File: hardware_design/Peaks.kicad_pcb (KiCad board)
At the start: 2 copper layers, 86.4 x 69.8 mm, 54 parts, among them J3 Eurorack Power, J8 Conn_01x07, Q1 2N3904, Q2 2N3904, U1 TL074, U2 Bluepill, U3 78l05

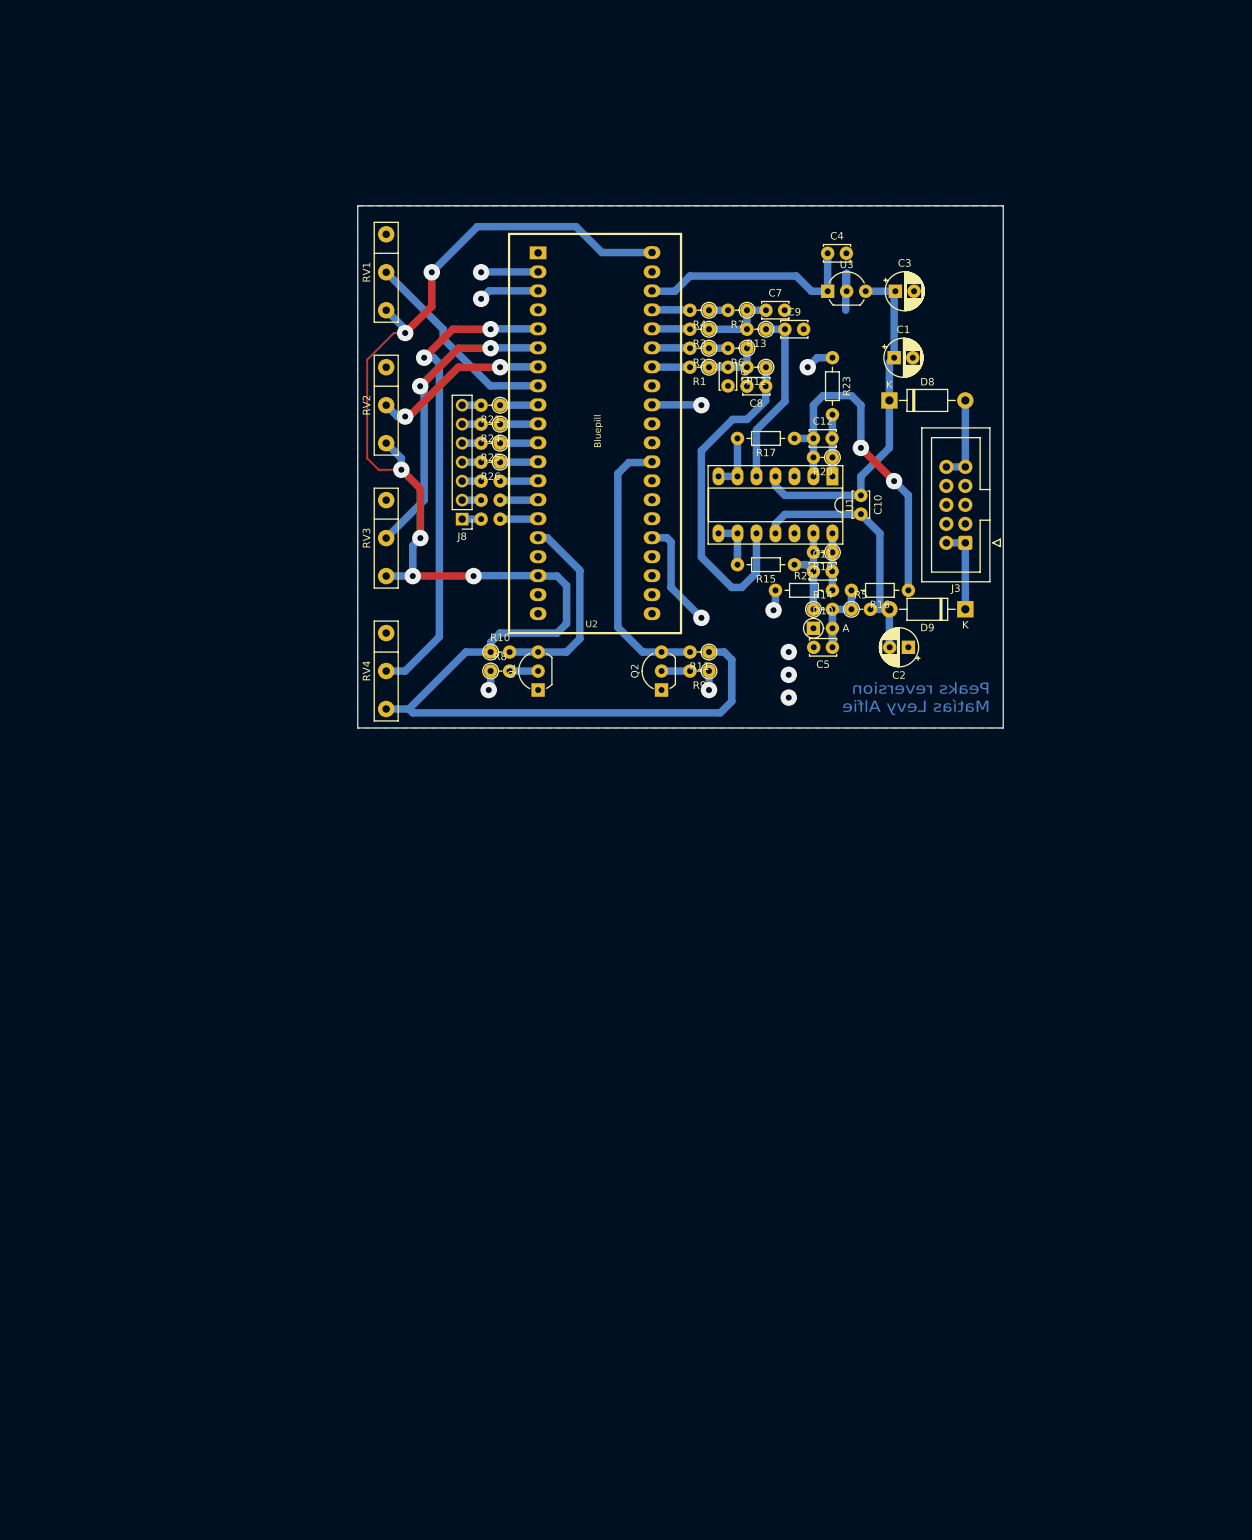
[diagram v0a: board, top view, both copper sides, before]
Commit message: update my KOSMO adaption
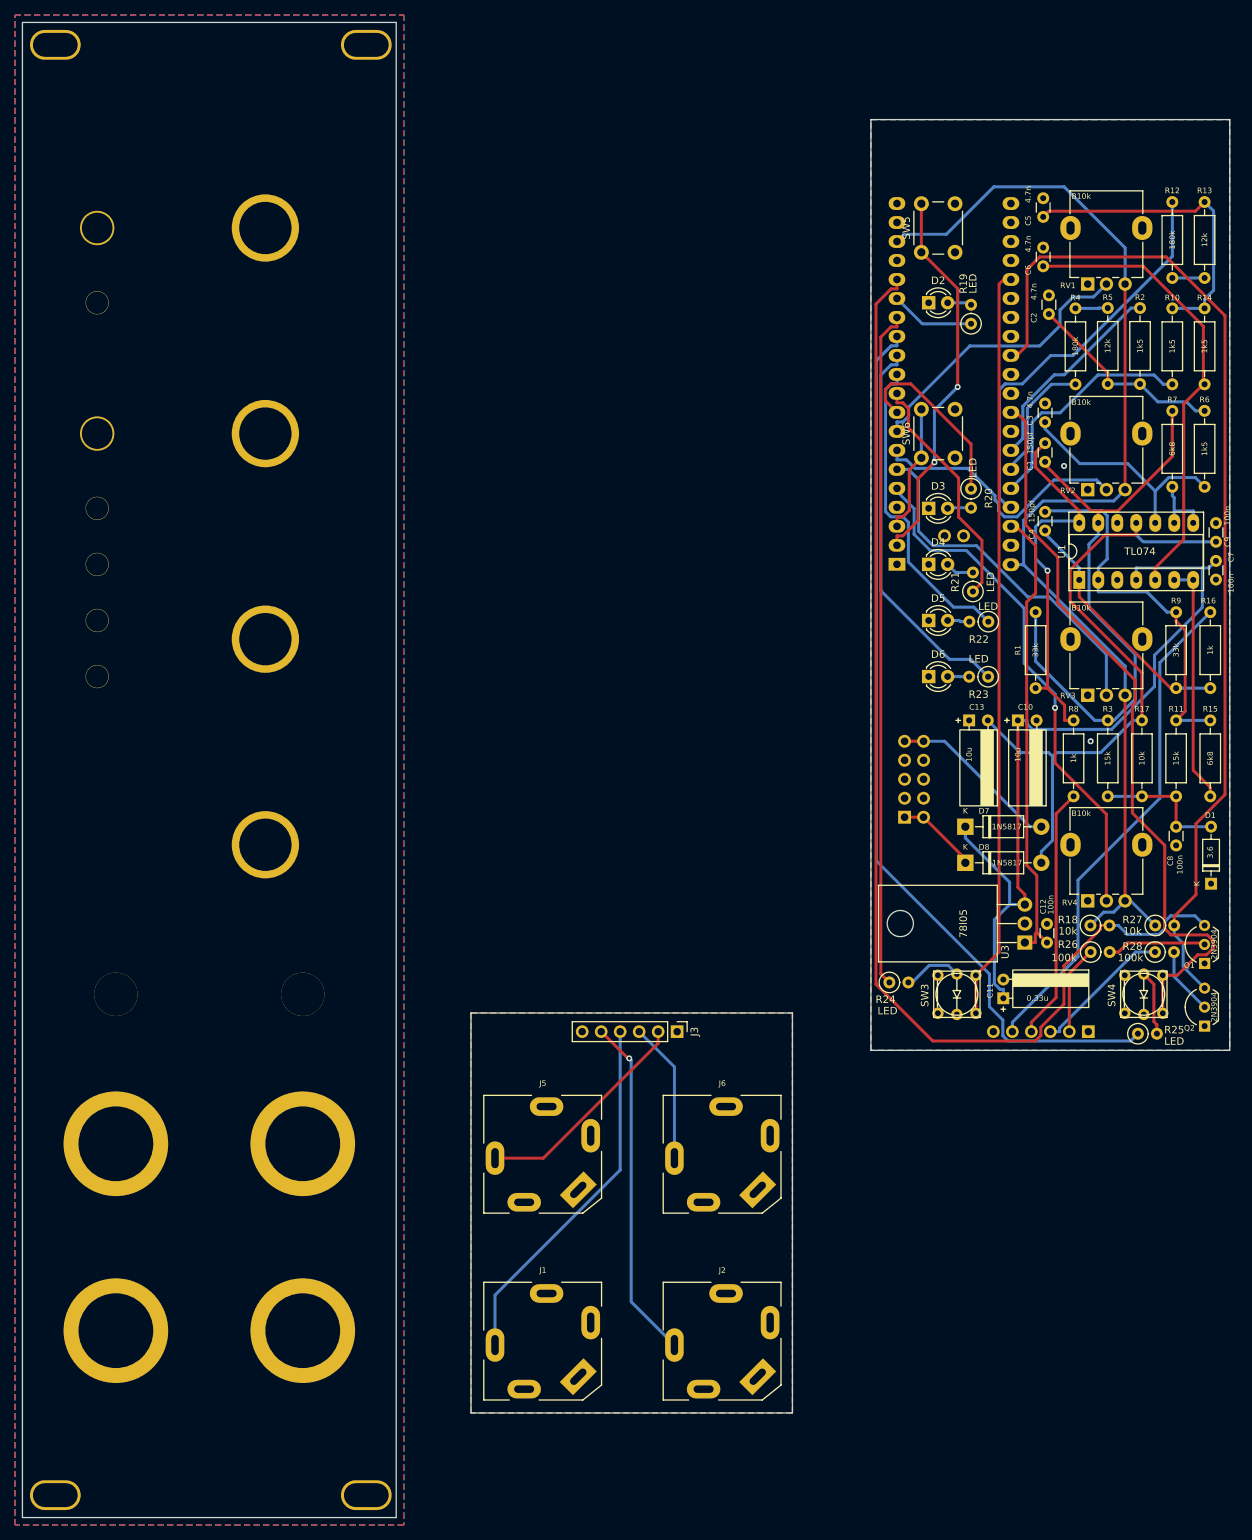
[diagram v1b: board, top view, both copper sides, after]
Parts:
- removed J8: Conn_01x07, Connector_PinHeader_2.54mm:PinHeader_1x07_P2.54mm_Vertical
- added C9: 100n, ao_tht:C_Disc_D3.0mm_W1.6mm_P2.50mm, F.Cu at (184.7, 94.5)
- added D2: LED, LED_THT:LED_D3.0mm_FlatTop, F.Cu at (146.2, 62.5)
- added D3: LED, LED_THT:LED_D3.0mm_FlatTop, F.Cu at (146.2, 90.0)
- added D4: LED, LED_THT:LED_D3.0mm_FlatTop, F.Cu at (146.2, 97.5)
- added D5: LED, LED_THT:LED_D3.0mm_FlatTop, F.Cu at (146.2, 105.0)
- added D6: LED, LED_THT:LED_D3.0mm_FlatTop, F.Cu at (146.2, 112.5)
- added G***: LOGO, panel:panel, F.Cu at (50.0, 125.0)
- added H25: led, Kosmo_panel:Kosmo_HIGHLY_PB6149L, F.Cu at (62.5, 155.0)
- added H25: led, Kosmo_panel:Kosmo_HIGHLY_PB6149L, F.Cu at (37.5, 155.0)
- added J1: out1, ao_tht:Jack_6.35mm_PJ_629HAN_slots, F.Cu at (94.6, 201.4)
- added J2: out2, ao_tht:Jack_6.35mm_PJ_629HAN_slots, F.Cu at (118.6, 201.4)
- added J4: Conn_01x06_Female, Connector_PinSocket_2.54mm:PinSocket_1x06_P2.54mm_Vertical, B.Cu at (167.6, 160.0)
- added J5: in1, ao_tht:Jack_6.35mm_PJ_629HAN_slots, F.Cu at (94.6, 176.4)
- added J6: in2, ao_tht:Jack_6.35mm_PJ_629HAN_slots, F.Cu at (118.6, 176.4)
- added J7: Synth_power_2x5, ao_tht:Power_Header, B.Cu at (143.0, 131.3)
- added REF**: Kosmo_Jack_Hole, Kosmo_panel:Kosmo_Jack_Hole, F.Cu at (62.5, 175.0)
- added REF**: 3mm_flat_LED, Kosmo_panel:Kosmo_LED_3mm, F.Cu at (35.0, 105.0)
- added REF**: 3mm_flat_LED, Kosmo_panel:Kosmo_LED_3mm, F.Cu at (35.0, 90.0)
- added REF**: 3mm_flat_LED, Kosmo_panel:Kosmo_LED_3mm, F.Cu at (35.0, 62.5)
- added REF**: Kosmo_Panel_Dual_Slotted_Mounting_Holes, Kosmo_panel:Kosmo_Panel_Dual_Slotted_Mounting_Holes, F.Cu at (28.0, 222.0)
- added REF**: Kosmo_Jack_Hole, Kosmo_panel:Kosmo_Jack_Hole, F.Cu at (37.5, 175.0)
- added REF**: Kosmo_LED_Hole, Kosmo_panel:Kosmo_LED_Hole, F.Cu at (35.0, 80.0)
- added REF**: Kosmo_Pot_Hole, Kosmo_panel:Kosmo_Pot_Hole, F.Cu at (57.5, 107.5)
- added REF**: Kosmo_Pot_Hole, Kosmo_panel:Kosmo_Pot_Hole, F.Cu at (57.5, 80.0)
- added REF**: Kosmo_Panel_Dual_Slotted_Mounting_Holes, Kosmo_panel:Kosmo_Panel_Dual_Slotted_Mounting_Holes, F.Cu at (69.6, 222.0)
- added REF**: Kosmo_Jack_Hole, Kosmo_panel:Kosmo_Jack_Hole, F.Cu at (37.5, 200.0)
- added REF**: Kosmo_LED_Hole, Kosmo_panel:Kosmo_LED_Hole, F.Cu at (35.0, 52.5)
- added REF**: Kosmo_Pot_Hole, Kosmo_panel:Kosmo_Pot_Hole, F.Cu at (57.5, 135.0)
- added REF**: 3mm_flat_LED, Kosmo_panel:Kosmo_LED_3mm, F.Cu at (35.0, 97.5)
- added REF**: Kosmo_Jack_Hole, Kosmo_panel:Kosmo_Jack_Hole, F.Cu at (62.5, 200.0)
- added REF**: Kosmo_Pot_Hole, Kosmo_panel:Kosmo_Pot_Hole, F.Cu at (57.5, 52.5)
- added REF**: 3mm_flat_LED, Kosmo_panel:Kosmo_LED_3mm, F.Cu at (35.0, 112.5)
- added SW3: TRIG_LED1, ao_tht:HIGHLY_PB6149L, F.Cu at (150.0, 155.0)
- added SW4: TRIG2_LED, ao_tht:HIGHLY_PB6149L, F.Cu at (175.0, 155.0)
- added SW5: SW_Push, Button_Switch_THT:SW_PUSH_6mm_H13mm, F.Cu at (145.2, 55.8)
- added SW6: SW_Push, Button_Switch_THT:SW_PUSH_6mm_H13mm, F.Cu at (145.2, 83.2)
- C1: renamed from C11; footprint Personal:C_Disc_D3.4mm_W2.1mm_P2.50mm_Large_Pads -> ao_tht:C_Disc_D3.0mm_W1.6mm_P2.50mm
- C10: renamed from C1; footprint Personal:CP_Radial_D5.0mm_P2.50mm_Large_Pads -> ao_tht:CP_Radial_horizontalflat_D5mm_P2.50mm_H10mm_south
- C11: renamed from C3; value 0,33u -> 0.33u; footprint Personal:CP_Radial_D5.0mm_P2.50mm_Large_Pads -> ao_tht:CP_Radial_horizontalflat_D5mm_P2.50mm_H10mm_south
- C12: renamed from C4; footprint Personal:C_Disc_D3.4mm_W2.1mm_P2.50mm_Large_Pads -> ao_tht:C_Disc_D3.0mm_W1.6mm_P2.50mm
- C13: renamed from C2; footprint Personal:CP_Radial_D5.0mm_P2.50mm_Large_Pads -> ao_tht:CP_Radial_horizontalflat_D5mm_P2.50mm_H10mm_south
- C2: renamed from C6; footprint Personal:C_Disc_D3.4mm_W2.1mm_P2.50mm_Large_Pads -> ao_tht:C_Disc_D3.0mm_W1.6mm_P2.50mm
- C3: renamed from C8; footprint Personal:C_Disc_D3.4mm_W2.1mm_P2.50mm_Large_Pads -> ao_tht:C_Disc_D3.0mm_W1.6mm_P2.50mm
- C4: renamed from C12; footprint Personal:C_Disc_D3.4mm_W2.1mm_P2.50mm_Large_Pads -> ao_tht:C_Disc_D3.0mm_W1.6mm_P2.50mm
- C5: renamed from C7; footprint Personal:C_Disc_D3.4mm_W2.1mm_P2.50mm_Large_Pads -> ao_tht:C_Disc_D3.0mm_W1.6mm_P2.50mm
- C6: renamed from C9; footprint Personal:C_Disc_D3.4mm_W2.1mm_P2.50mm_Large_Pads -> ao_tht:C_Disc_D3.0mm_W1.6mm_P2.50mm
- C7: renamed from C10; footprint Personal:C_Disc_D3.4mm_W2.1mm_P2.50mm_Large_Pads -> ao_tht:C_Disc_D3.0mm_W1.6mm_P2.50mm
- C8: renamed from C5; footprint Personal:C_Disc_D3.4mm_W2.1mm_P2.50mm_Large_Pads -> ao_tht:C_Disc_D3.0mm_W1.6mm_P2.50mm
- D1: renamed from D10; footprint Personal:D_DO-35_SOD27_P2.54mm_Vertical_AnodeUp_Large_Pads -> ao_tht:D_DO-35_SOD27_P7.62mm_Horizontal
- D7: renamed from D8; footprint Diode_THT:D_DO-41_SOD81_P10.16mm_Horizontal -> ao_tht:D_DO-41_SOD81_P10.16mm_Horizontal
- D8: renamed from D9; footprint Diode_THT:D_DO-41_SOD81_P10.16mm_Horizontal -> ao_tht:D_DO-41_SOD81_P10.16mm_Horizontal
- J3: value Eurorack Power -> Conn_01x06_Male; footprint Personal:IDC-Header_2x05_P2.54mm_Vertical_Large_Pads -> Connector_PinHeader_2.54mm:PinHeader_1x06_P2.54mm_Vertical
- Q1, Q2: footprint Personal:TO-92_Inline_Wide_Large_Pads -> ao_tht:TO-92_Inline_Wide
- R1: renamed from R19; footprint Personal:R_Axial_DIN0204_L3.6mm_D1.6mm_P2.54mm_Vertical_Large_Pads -> ao_tht:R_Axial_DIN0207_L6.3mm_D2.5mm_P10.16mm_Horizontal
- R10: renamed from R3; footprint Personal:R_Axial_DIN0204_L3.6mm_D1.6mm_P2.54mm_Vertical_Large_Pads -> ao_tht:R_Axial_DIN0207_L6.3mm_D2.5mm_P10.16mm_Horizontal
- R11: renamed from R16; footprint Personal:R_Axial_DIN0204_L3.6mm_D1.6mm_P7.62mm_Horizontal_Large_Pads -> ao_tht:R_Axial_DIN0207_L6.3mm_D2.5mm_P10.16mm_Horizontal
- R12: renamed from R4; footprint Personal:R_Axial_DIN0204_L3.6mm_D1.6mm_P2.54mm_Vertical_Large_Pads -> ao_tht:R_Axial_DIN0207_L6.3mm_D2.5mm_P10.16mm_Horizontal
- R13: renamed from R7; footprint Personal:R_Axial_DIN0204_L3.6mm_D1.6mm_P2.54mm_Vertical_Large_Pads -> ao_tht:R_Axial_DIN0207_L6.3mm_D2.5mm_P10.16mm_Horizontal
- R14: renamed from R13; footprint Personal:R_Axial_DIN0204_L3.6mm_D1.6mm_P2.54mm_Vertical_Large_Pads -> ao_tht:R_Axial_DIN0207_L6.3mm_D2.5mm_P10.16mm_Horizontal
- R15: renamed from R17; footprint Personal:R_Axial_DIN0204_L3.6mm_D1.6mm_P7.62mm_Horizontal_Large_Pads -> ao_tht:R_Axial_DIN0207_L6.3mm_D2.5mm_P10.16mm_Horizontal
- R16: renamed from R23; footprint Personal:R_Axial_DIN0204_L3.6mm_D1.6mm_P7.62mm_Horizontal_Large_Pads -> ao_tht:R_Axial_DIN0207_L6.3mm_D2.5mm_P10.16mm_Horizontal
- R17: renamed from R5; footprint Personal:R_Axial_DIN0204_L3.6mm_D1.6mm_P2.54mm_Vertical_Large_Pads -> ao_tht:R_Axial_DIN0207_L6.3mm_D2.5mm_P10.16mm_Horizontal
- R18: renamed from R10; footprint Personal:R_Axial_DIN0204_L3.6mm_D1.6mm_P2.54mm_Vertical_Large_Pads -> ao_tht:R_Axial_DIN0207_L6.3mm_D2.5mm_P2.54mm_Vertical
- R19: renamed from R18; value 2k -> LED; footprint Personal:R_Axial_DIN0204_L3.6mm_D1.6mm_P2.54mm_Vertical_Large_Pads -> ao_tht:R_Axial_DIN0207_L6.3mm_D2.5mm_P2.54mm_Vertical; moved to F.Cu
- R2: renamed from R1; footprint Personal:R_Axial_DIN0204_L3.6mm_D1.6mm_P2.54mm_Vertical_Large_Pads -> ao_tht:R_Axial_DIN0207_L6.3mm_D2.5mm_P10.16mm_Horizontal
- R20: renamed from R21; value 2k -> LED; footprint Personal:R_Axial_DIN0204_L3.6mm_D1.6mm_P2.54mm_Vertical_Large_Pads -> ao_tht:R_Axial_DIN0207_L6.3mm_D2.5mm_P2.54mm_Vertical
- R21: renamed from R24; value 2k -> LED; footprint Personal:R_Axial_DIN0204_L3.6mm_D1.6mm_P2.54mm_Vertical_Large_Pads -> ao_tht:R_Axial_DIN0207_L6.3mm_D2.5mm_P2.54mm_Vertical
- R22: renamed from R25; value 2k -> LED; footprint Personal:R_Axial_DIN0204_L3.6mm_D1.6mm_P2.54mm_Vertical_Large_Pads -> ao_tht:R_Axial_DIN0207_L6.3mm_D2.5mm_P2.54mm_Vertical
- R23: renamed from R26; value 2k -> LED; footprint Personal:R_Axial_DIN0204_L3.6mm_D1.6mm_P2.54mm_Vertical_Large_Pads -> ao_tht:R_Axial_DIN0207_L6.3mm_D2.5mm_P2.54mm_Vertical
- R24: renamed from R27; value 2k -> LED; footprint Personal:R_Axial_DIN0204_L3.6mm_D1.6mm_P2.54mm_Vertical_Large_Pads -> ao_tht:R_Axial_DIN0207_L6.3mm_D2.5mm_P2.54mm_Vertical; moved to F.Cu
- R25: renamed from R28; value 2k -> LED; footprint Personal:R_Axial_DIN0204_L3.6mm_D1.6mm_P2.54mm_Vertical_Large_Pads -> ao_tht:R_Axial_DIN0207_L6.3mm_D2.5mm_P2.54mm_Vertical; moved to F.Cu
- R26: renamed from R8; footprint Personal:R_Axial_DIN0204_L3.6mm_D1.6mm_P2.54mm_Vertical_Large_Pads -> ao_tht:R_Axial_DIN0207_L6.3mm_D2.5mm_P2.54mm_Vertical
- R27: renamed from R11; footprint Personal:R_Axial_DIN0204_L3.6mm_D1.6mm_P2.54mm_Vertical_Large_Pads -> ao_tht:R_Axial_DIN0207_L6.3mm_D2.5mm_P2.54mm_Vertical
- R28: renamed from R9; footprint Personal:R_Axial_DIN0204_L3.6mm_D1.6mm_P2.54mm_Vertical_Large_Pads -> ao_tht:R_Axial_DIN0207_L6.3mm_D2.5mm_P2.54mm_Vertical
- R3: renamed from R14; footprint Personal:R_Axial_DIN0204_L3.6mm_D1.6mm_P2.54mm_Vertical_Large_Pads -> ao_tht:R_Axial_DIN0207_L6.3mm_D2.5mm_P10.16mm_Horizontal
- R4: renamed from R2; footprint Personal:R_Axial_DIN0204_L3.6mm_D1.6mm_P2.54mm_Vertical_Large_Pads -> ao_tht:R_Axial_DIN0207_L6.3mm_D2.5mm_P10.16mm_Horizontal
- R5: renamed from R6; footprint Personal:R_Axial_DIN0204_L3.6mm_D1.6mm_P2.54mm_Vertical_Large_Pads -> ao_tht:R_Axial_DIN0207_L6.3mm_D2.5mm_P10.16mm_Horizontal
- R6: renamed from R12; footprint Personal:R_Axial_DIN0204_L3.6mm_D1.6mm_P2.54mm_Vertical_Large_Pads -> ao_tht:R_Axial_DIN0207_L6.3mm_D2.5mm_P10.16mm_Horizontal
- R7: renamed from R15; footprint Personal:R_Axial_DIN0204_L3.6mm_D1.6mm_P7.62mm_Horizontal_Large_Pads -> ao_tht:R_Axial_DIN0207_L6.3mm_D2.5mm_P10.16mm_Horizontal
- R8: renamed from R22; footprint Personal:R_Axial_DIN0204_L3.6mm_D1.6mm_P7.62mm_Horizontal_Large_Pads -> ao_tht:R_Axial_DIN0207_L6.3mm_D2.5mm_P10.16mm_Horizontal
- R9: renamed from R20; footprint Personal:R_Axial_DIN0204_L3.6mm_D1.6mm_P2.54mm_Vertical_Large_Pads -> ao_tht:R_Axial_DIN0207_L6.3mm_D2.5mm_P10.16mm_Horizontal
- RV1, RV2, RV3, RV4: footprint Personal:Potenciometro -> ao_tht:Potentiometer_Alpha_RD901F-40-00D_Single_Vertical_centered
- U2: footprint BluePill_breakouts:BluePill_STM32F103C -> ao_tht:BluePill_STM32F103C; moved to B.Cu
- U3: footprint Personal:TO-92_Inline_Wide_Large_Pads -> Package_TO_SOT_THT:TO-220-3_Horizontal_TabDown
- moved R25 112.9 mm to (174.2, 160.3), turned to 0 degrees
- moved RV4 99.1 mm to (170.0, 135.0), turned to 90 degrees
- moved RV3 97.3 mm to (170.0, 107.5), turned to 90 degrees
- moved C12 96.8 mm to (162.1, 148.1), turned to 90 degrees
- moved RV1 96.5 mm to (170.0, 52.5), turned to 90 degrees
- moved RV2 96.4 mm to (170.0, 80.0), turned to 90 degrees
- moved Q1 96.4 mm to (183.1, 150.9)
- moved C11 95.7 mm to (156.2, 155.5), turned to 90 degrees
- moved U3 91.0 mm to (159.1, 148.1), turned to 90 degrees
- moved R26 88.6 mm to (167.9, 149.4)
- moved R18 88.2 mm to (167.9, 145.8)
- moved Q2 85.4 mm to (183.1, 159.3)
- moved R24 82.9 mm to (141.0, 153.4), turned to 0 degrees
- moved J3 75.9 mm to (112.6, 160.0), turned to -90 degrees
- moved R23 71.3 mm to (154.2, 112.5)
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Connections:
- C7 pad 2: -12V -> GND
- D7 pad 2: Net-(D8-Pad2) -> Net-(D7-Pad2)
- D8 pad 1: Net-(D9-Pad1) -> Net-(D8-Pad1)
- J3 pad 1: Net-(D9-Pad1) -> GND
- J3 pad 2: Net-(D9-Pad1) -> FROM_IN1
- J3 pad 3: GND -> FROM_IN2
- J3 pad 4: GND -> FROM_OUT1
- J3 pad 5: GND -> FROM_OUT2
- R19 pad 2: TO_D1 -> Net-(D2-Pad2)
- R20 pad 2: TO_D2 -> Net-(D3-Pad2)
- R21 pad 2: TO_D3 -> Net-(D4-Pad2)
- R22 pad 2: TO_D4 -> Net-(D5-Pad2)
- R23 pad 2: TO_D5 -> Net-(D6-Pad2)
- R24 pad 2: TO_D6 -> Net-(R24-Pad2)
- R25 pad 2: TO_D7 -> Net-(R25-Pad2)
- U2 pad 1: Net-(U2-Pad1) -> unconnected-(U2-Pad1)
- U2 pad 17: Net-(U2-Pad17) -> unconnected-(U2-Pad17)
- U2 pad 21: Net-(U2-Pad21) -> unconnected-(U2-Pad21)
- U2 pad 22: Net-(U2-Pad22) -> unconnected-(U2-Pad22)
- U2 pad 23: Net-(U2-Pad23) -> unconnected-(U2-Pad23)
- U2 pad 24: Net-(U2-Pad24) -> unconnected-(U2-Pad24)
- U2 pad 26: Net-(U2-Pad26) -> unconnected-(U2-Pad26)
- U2 pad 27: Net-(U2-Pad27) -> unconnected-(U2-Pad27)
- U2 pad 28: Net-(U2-Pad28) -> unconnected-(U2-Pad28)
- U2 pad 30: Net-(U2-Pad30) -> unconnected-(U2-Pad30)
- U2 pad 31: Net-(U2-Pad31) -> unconnected-(U2-Pad31)
- U2 pad 33: Net-(U2-Pad33) -> unconnected-(U2-Pad33)
- U2 pad 4: Net-(U2-Pad4) -> unconnected-(U2-Pad4)
- U2 pad 41: Net-(U2-Pad41) -> unconnected-(U2-Pad41)
- U2 pad 42: Net-(U2-Pad42) -> unconnected-(U2-Pad42)
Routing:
- net /TRIG_1: track 26.7 -> 156.0 mm
- net /LED_SALIDA_2: track 5.10 -> 120.9 mm
- net /TRIG_2: track 36.8 -> 137.7 mm
- net /SW_TRIG2: track 6.63 -> 99.8 mm, vias 1 -> 0
- net /SW_TRIG1: track 14.6 -> 100.7 mm, vias 1 -> 0
- net /LED_SALIDA_1: track 5.10 -> 90.8 mm
- net Net-(C1-Pad1): track 13.1 -> 81.7 mm
- net TO_OUT2: track 3.83 -> 67.1 mm, vias 1 -> 0
- net +12V: track 46.4 -> 106.6 mm
- net -12V: track 35.9 -> 88.6 mm
- net +3V3: track 204.6 -> 154.2 mm, vias 6 -> 0
- net /CH2_PWM2: track 5.10 -> 54.3 mm
- net FROM_OUT1: track 0.00 -> 48.9 mm
- net /LED5: track 5.10 -> 51.9 mm
- net FROM_OUT2: track 0.00 -> 46.1 mm, vias 0 -> 1
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- added copper zone on F.Cu, net GND
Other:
- board size 86.4 x 69.8 mm -> 161.5 x 200 mm
- net class Default removed
- rule pad_to_mask_clearance: 0.05 -> 0
- board text added: "JLCJLCJLCJLC"
- board text removed: "Peaks reversion Matías Levy Alfie"
